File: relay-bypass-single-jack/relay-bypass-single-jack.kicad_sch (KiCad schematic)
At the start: 49 parts, among them J1 3, J2 TC2030, J5 Conn_Coaxial_Small, Q1 DMP3099L, Q2 DMN62D0U-7, U1 TLV76701DRVR, U2 STM32C011F4Ux

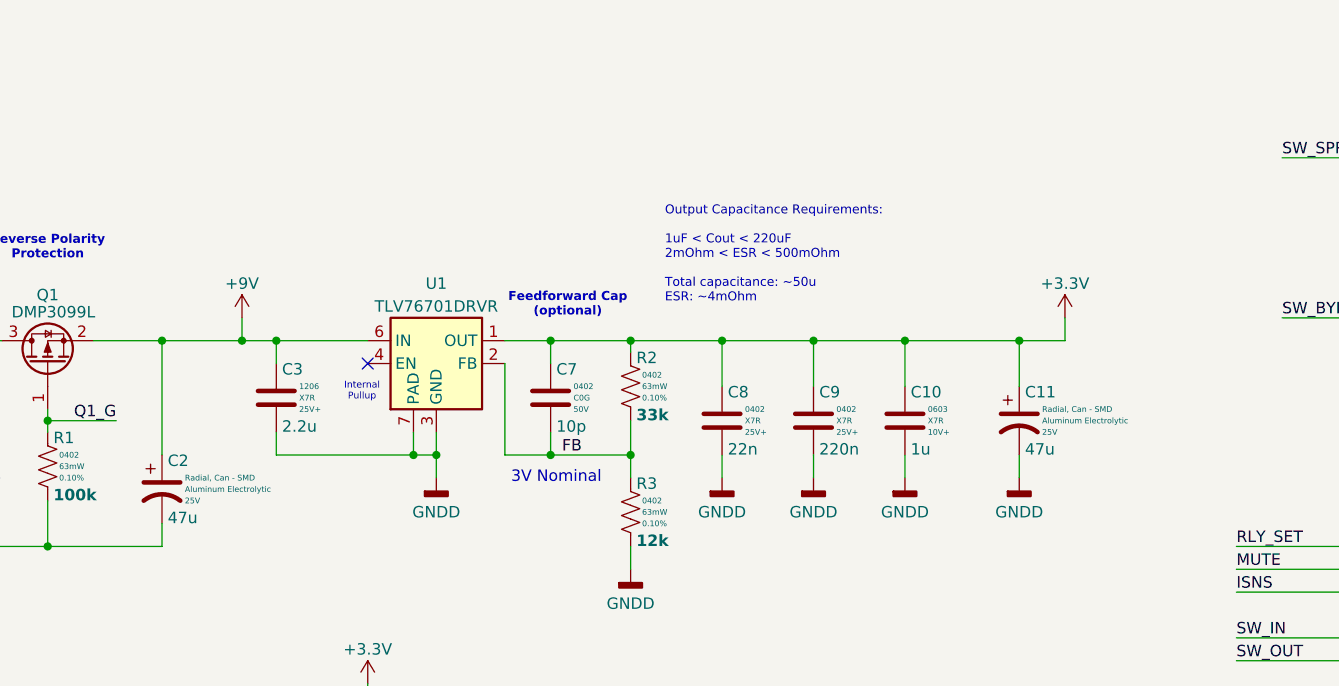
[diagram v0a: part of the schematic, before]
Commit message: Scratchwork
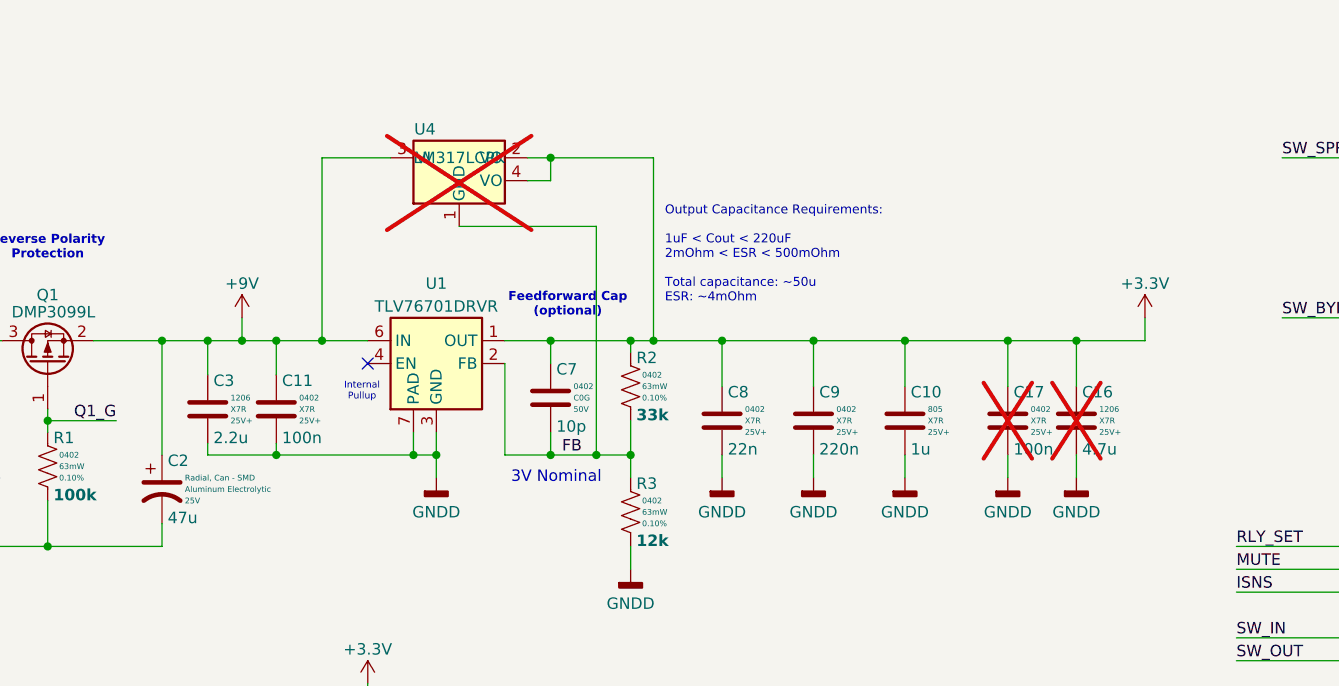
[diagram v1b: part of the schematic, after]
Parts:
- removed C11: 47u, Capacitor_SMD:CP_Elec_6.3x5.8, symbol #gplm:cap/CAP-3005-047U
- added C11, C17: 100n, Capacitor_SMD:C_0402_1005Metric, symbol #gplm:cap/CAP-4103-100N
- added C16: 4.7u, Capacitor_SMD:C_1206_3216Metric, symbol #gplm:cap/CAP-4106-04U7
- added U4: LM317LCPK, Package_TO_SOT_SMD:SOT-223, symbol #gplm:reg/REG-1011-0ADJ
- C10: footprint Capacitor_SMD:C_0603_1608Metric -> Capacitor_SMD:C_0805_2012Metric; symbol #gplm:cap/CAP-4107-001U -> #gplm:cap/CAP-4105-001U; IPN CAP-4107-001U -> CAP-4105-001U; MPN C0603C105K8RACTU -> C0805C105K3RACTU; Package/Case 0603 -> 805; Voltage 10V+ -> 25V+
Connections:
- net +3.3V: now also C16.1, C17.1, U4.2 (VO), U4.4 (VO)
- net +9V: now also C11.1, U4.3 (VI)
- net FB: now also U4.1 (GND)
- net GNDD: now also C11.2, C16.2, C17.2
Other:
- moved on the sheet: C3
